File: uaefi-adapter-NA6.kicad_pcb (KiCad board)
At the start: 2 copper layers, 1 part

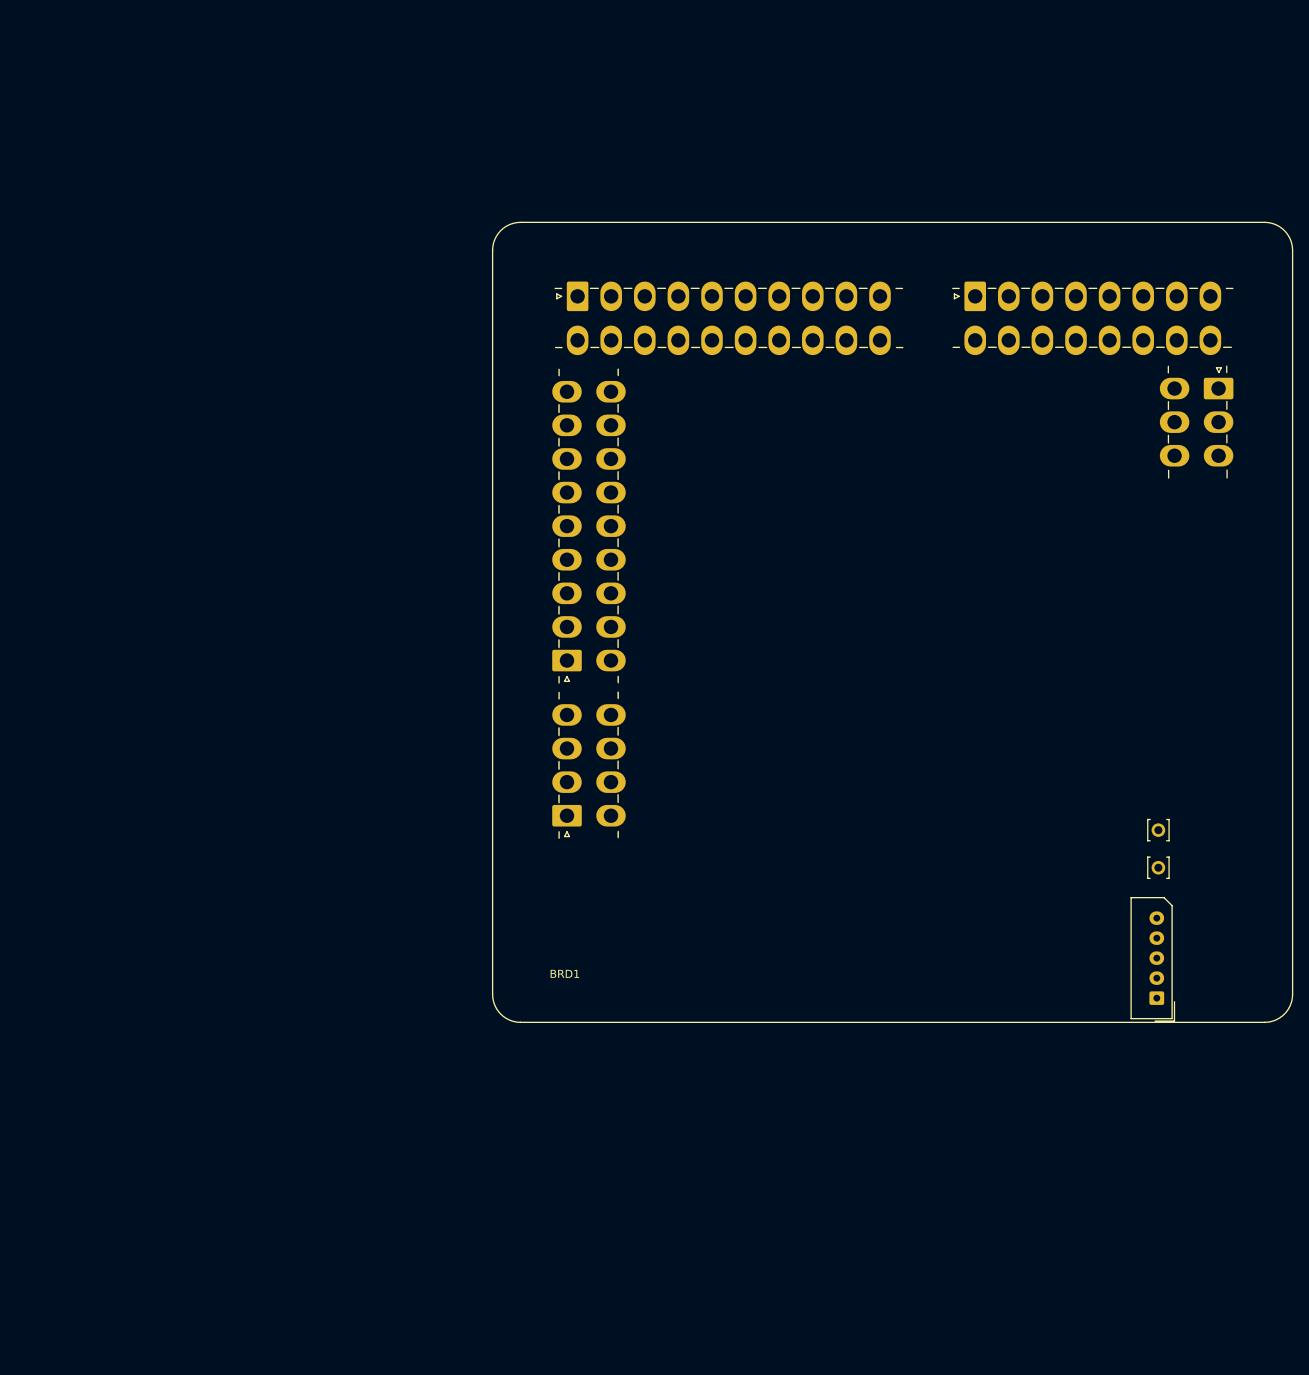
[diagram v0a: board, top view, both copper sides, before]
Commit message: upd
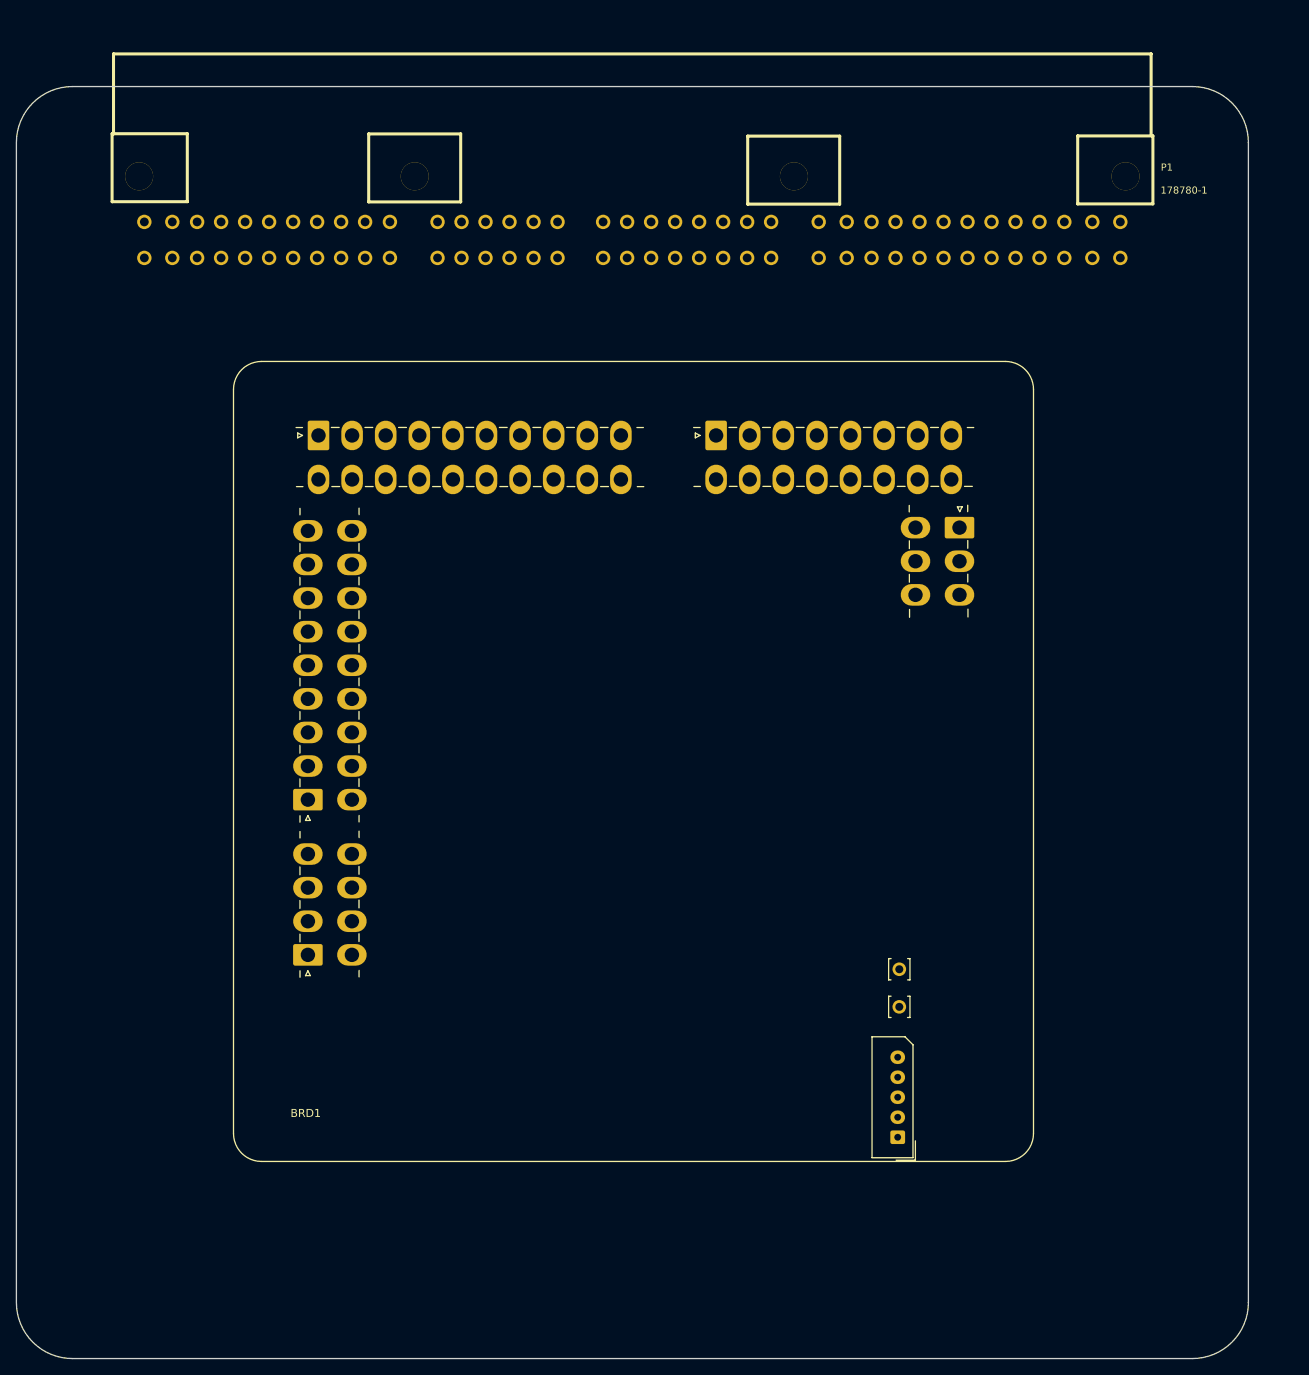
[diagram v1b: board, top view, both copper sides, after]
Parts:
- added P1: 178780-1, hellen-one-common:178780-1, F.Cu at (146.0, 47.0)
- moved BRD1 36.8 mm to (47.6, 159.9)
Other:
- board outline added: 154 x 159 mm

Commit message: upd
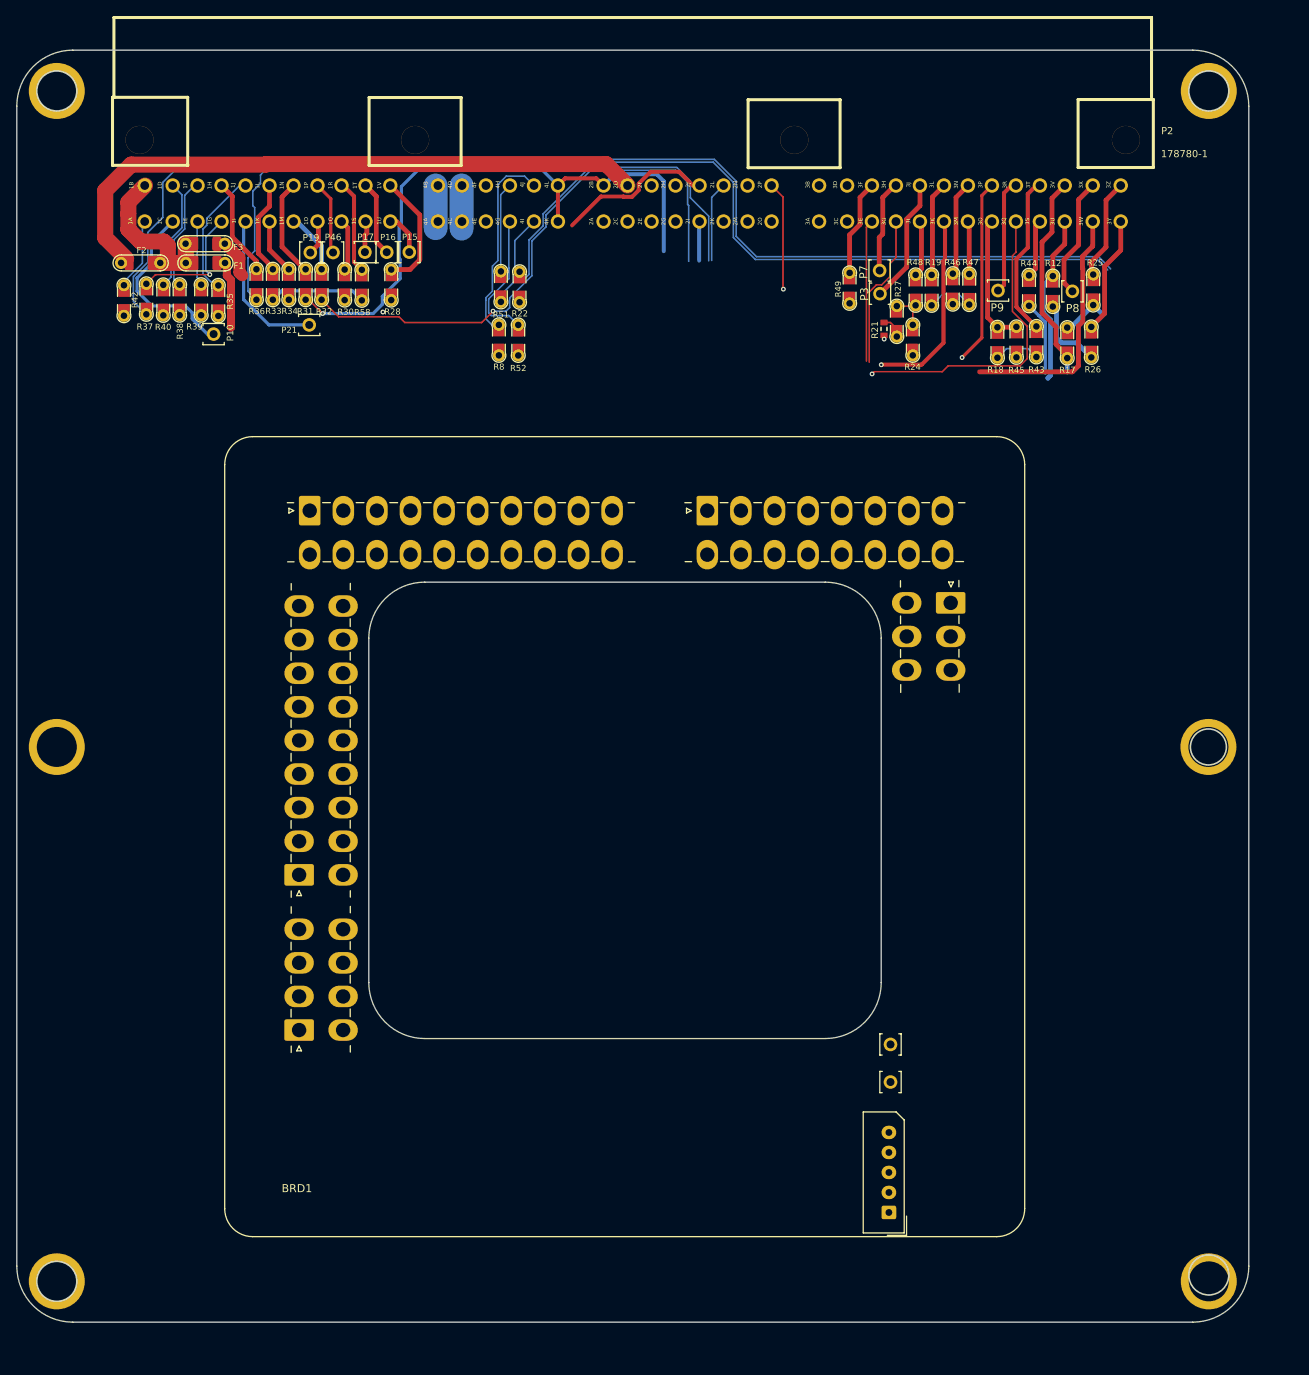
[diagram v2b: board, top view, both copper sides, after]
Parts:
- removed P1: 178780-1, hellen-one-common:178780-1
- added F1: Fuse-Pad-Pad, hellen-one-common:PAD-1206-PAD, F.Cu at (44.1, 47.6)
- added F2: Fuse-Pad-Pad, hellen-one-common:PAD-1206-PAD, F.Cu at (36.0, 47.6)
- added F3: Fuse-Pad-Pad, hellen-one-common:PAD-1206-PAD, F.Cu at (44.1, 45.2)
- added J11: Conn_01x01, MountingHole:MountingHole_4.5mm_Pad, F.Cu at (25.5, 26.1)
- added J13: Conn_01x01, MountingHole:MountingHole_4.5mm_Pad, F.Cu at (25.5, 174.9)
- added J14: Conn_01x01, MountingHole:MountingHole_4.5mm_Pad, F.Cu at (169.5, 174.9)
- added J15: Conn_01x01, MountingHole:MountingHole_4.5mm_Pad, F.Cu at (169.5, 108.1)
- added J16: Conn_01x01, MountingHole:MountingHole_4.5mm_Pad, F.Cu at (169.5, 26.1)
- added J17: Conn_01x01, MountingHole:MountingHole_4.5mm_Pad, F.Cu at (25.5, 108.1)
- added P10: Pad, hellen-one-common:PAD-TH, F.Cu at (45.1, 56.5)
- added P15: Pad, hellen-one-common:PAD-TH, F.Cu at (69.6, 46.2)
- added P16: Pad, hellen-one-common:PAD-TH, F.Cu at (66.7, 46.3)
- added P17: Pad, hellen-one-common:PAD-TH, F.Cu at (64.0, 46.2)
- added P19: Pad, hellen-one-common:PAD-TH, F.Cu at (57.2, 46.3)
- added P2: 178780-1, hellen-one-common:178780-1, F.Cu at (146.0, 42.4)
- added P21: Pad, hellen-one-common:PAD-TH, F.Cu at (57.1, 55.3)
- added P3: Pad, hellen-one-common:PAD-TH, F.Cu at (128.4, 51.4)
- added P46: Pad, hellen-one-common:PAD-TH, F.Cu at (60.0, 46.3)
- added P7: Pad, hellen-one-common:PAD-TH, F.Cu at (128.4, 48.5)
- added P8: Pad, hellen-one-common:PAD-TH, F.Cu at (152.5, 51.1)
- added P9: Pad, hellen-one-common:PAD-TH, F.Cu at (143.2, 51.0)
- added R12: Jumper-Pad-Pad, hellen-one-common:PAD-0805-PAD, F.Cu at (150.0, 51.1)
- added R17: Jumper-Pad-Pad, hellen-one-common:PAD-0805-PAD, F.Cu at (151.8, 57.6)
- added R18: Jumper-Pad-Pad, hellen-one-common:PAD-0805-PAD, F.Cu at (143.1, 57.5)
- added R19: Jumper-Pad-Pad, hellen-one-common:PAD-0805-PAD, F.Cu at (134.9, 51.0)
- added R21: 1k, hellen-one-common:R0603, F.Cu at (128.9, 55.8)
- added R22: Jumper-Pad-Pad, hellen-one-common:PAD-0805-PAD, F.Cu at (83.3, 50.6)
- added R24: Jumper-Pad-Pad, hellen-one-common:PAD-0805-PAD, F.Cu at (132.5, 57.2)
- added R25: Jumper-Pad-Pad, hellen-one-common:PAD-0805-PAD, F.Cu at (155.1, 51.0)
- added R26: Jumper-Pad-Pad, hellen-one-common:PAD-0805-PAD, F.Cu at (154.8, 57.5)
- added R27: Jumper-Pad-Pad, hellen-one-common:PAD-0805-PAD, F.Cu at (130.5, 54.9)
- added R28: Jumper-Pad-Pad, hellen-one-common:PAD-0805-PAD, F.Cu at (67.3, 50.3)
- added R30: Jumper-Pad-Pad, hellen-one-common:PAD-0805-PAD, F.Cu at (61.5, 50.3)
- added R31: Jumper-Pad-Pad, hellen-one-common:PAD-0805-PAD, F.Cu at (56.6, 50.3)
- added R32: Jumper-Pad-Pad, hellen-one-common:PAD-0805-PAD, F.Cu at (58.6, 50.3)
- added R33: Jumper-Pad-Pad, hellen-one-common:PAD-0805-PAD, F.Cu at (52.5, 50.3)
- added R34: Jumper-Pad-Pad, hellen-one-common:PAD-0805-PAD, F.Cu at (54.5, 50.3)
- added R35: Jumper-Pad-Pad, hellen-one-common:PAD-0805-PAD, F.Cu at (45.7, 52.3)
- added R36: Jumper-Pad-Pad, hellen-one-common:PAD-0805-PAD, F.Cu at (50.5, 50.3)
- added R37: Jumper-Pad-Pad, hellen-one-common:PAD-0805-PAD, F.Cu at (36.7, 52.1)
- added R38: Jumper-Pad-Pad, hellen-one-common:PAD-0805-PAD, F.Cu at (40.9, 52.2)
- added R39: Jumper-Pad-Pad, hellen-one-common:PAD-0805-PAD, F.Cu at (43.5, 52.2)
- added R40: Jumper-Pad-Pad, hellen-one-common:PAD-0805-PAD, F.Cu at (38.8, 52.2)
- added R42: Jumper-Pad-Pad, hellen-one-common:PAD-0805-PAD, F.Cu at (33.9, 52.3)
- added R43: Jumper-Pad-Pad, hellen-one-common:PAD-0805-PAD, F.Cu at (148.0, 57.4)
- added R44: Jumper-Pad-Pad, hellen-one-common:PAD-0805-PAD, F.Cu at (147.0, 51.0)
- added R45: Jumper-Pad-Pad, hellen-one-common:PAD-0805-PAD, F.Cu at (145.5, 57.5)
- added R46: Jumper-Pad-Pad, hellen-one-common:PAD-0805-PAD, F.Cu at (137.5, 50.8)
- added R47: Jumper-Pad-Pad, hellen-one-common:PAD-0805-PAD, F.Cu at (139.6, 50.9)
- added R48: Jumper-Pad-Pad, hellen-one-common:PAD-0805-PAD, F.Cu at (132.9, 51.0)
- added R49: Jumper-Pad-Pad, hellen-one-common:PAD-0805-PAD, F.Cu at (124.6, 50.7)
- added R51: Jumper-Pad-Pad, hellen-one-common:PAD-0805-PAD, F.Cu at (81.0, 50.6)
- added R52: Jumper-Pad-Pad, hellen-one-common:PAD-0805-PAD, F.Cu at (83.2, 57.3)
- added R58: Jumper-Pad-Pad, hellen-one-common:PAD-0805-PAD, F.Cu at (63.6, 50.4)
- added R8: Jumper-Pad-Pad, hellen-one-common:PAD-0805-PAD, F.Cu at (80.8, 57.2)
- moved BRD1 9.46 mm to (46.5, 169.3)
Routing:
- net (no net): track 0.00 -> 1371.6 mm, vias 0 -> 9
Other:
- outline, holes or cut-outs redrawn
- board text added: "+"
- board text added: "+5V"
- board text added: "+5VA"
- board text added: "-"
- board text added: "12_PERM"
- board text added: "12_RAW"
- board text added: "1A"
- board text added: "1B"
- board text added: "1C"
- board text added: "1D"
- board text added: "1E"
- board text added: "1F"
- board text added: "1G"
- board text added: "1H"
- board text added: "1I"
- board text added: "1J"
- board text added: "1K"
- board text added: "1L"
- board text added: "1M"
- board text added: "1N"
- board text added: "1O"
- board text added: "1P"
- board text added: "1Q"
- board text added: "1R"
- board text added: "1S"
- board text added: "1T"
- board text added: "1U"
- board text added: "1V"
- board text added: "2A"
- board text added: "2B"
- board text added: "2C"
- board text added: "2D"
- board text added: "2E"
- board text added: "2F"
- board text added: "2G"
- board text added: "2H"
- board text added: "2I"
- board text added: "2J"
- board text added: "2K"
- board text added: "2L"
- board text added: "2M"
- board text added: "2N"
- board text added: "2O"
- board text added: "2P"
- board text added: "3A"
- board text added: "3B"
- board text added: "3C"
- board text added: "3D"
- board text added: "3E"
- board text added: "3F"
- board text added: "3G"
- board text added: "3H"
- board text added: "3I"
- board text added: "3J"
- board text added: "3K"
- board text added: "3L"
- board text added: "3M"
- board text added: "3N"
- board text added: "3O"
- board text added: "3P"
- board text added: "3Q"
- board text added: "3R"
- board text added: "3S"
- board text added: "3T"
- board text added: "3U"
- board text added: "3V"
- board text added: "3W"
- board text added: "3X"
- board text added: "3Y"
- board text added: "3Z"
- board text added: "4A"
- board text added: "4B"
- board text added: "4C"
- board text added: "4D"
- board text added: "4E"
- board text added: "4F"
- board text added: "4G"
- board text added: "4H"
- board text added: "4I"
- board text added: "4J"
- board text added: "4K"
- board text added: "4L"
- board text added: "5VTPS"
- board text added: "A/C"
- board text added: "AFR"
- board text added: "BOOST"
- board text added: "CAM"
- board text added: "CAN_H"
- board text added: "CAN_L"
- board text added: "CFAN"
- board text added: "CLT"
- board text added: "CLUTCH"
- board text added: "CRANK"
- board text added: "DIGITAL"
- board text added: "ECF"
- board text added: "ETB"
- board text added: "GND"
- board text added: "H+"
- board text added: "H-"
- board text added: "IAT"
- board text added: "IDLE"
- board text added: "IGN2"
- board text added: "INJ1"
- board text added: "INJ2"
- board text added: "INJ3"
- board text added: "INJ4"
- board text added: "IP"
- board text added: "KNOCK"
- board text added: "MAF"
- board text added: "PPS1"
- board text added: "PPS2"
- board text added: "PRESSURE"
- board text added: "PUMP"
- board text added: "RTrim"
- board text added: "TACH"
- board text added: "TEMP"
- board text added: "TPS"
- board text added: "TPS1"
- board text added: "TPS2"
- board text added: "VS"
- board text added: "VS/IP"
- board text added: "VSS"
- board text added: "VVT"
- board text added: "WBO"
